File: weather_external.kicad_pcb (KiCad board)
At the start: 2 copper layers, 36 x 76 mm, 19 parts, among them J1 Conn_01x06_Male, J2 Conn_01x02_Male, J3 Conn_01x03_Male, J4 Conn_01x04_Male, Q1 IRF510PBF, SW1 SW_Push, U1 MCP1700-3302E_SOT23, U3 NE555DR

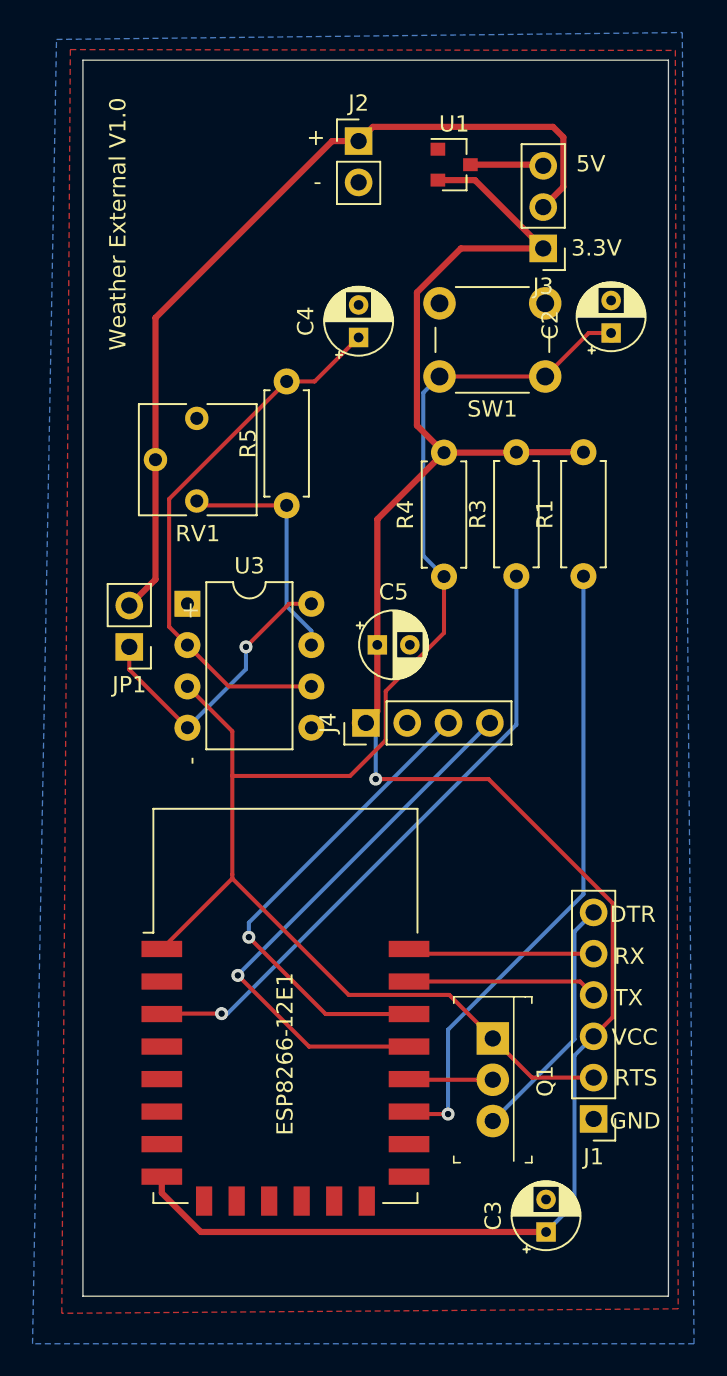
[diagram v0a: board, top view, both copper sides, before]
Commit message: Version 1.2. Small components
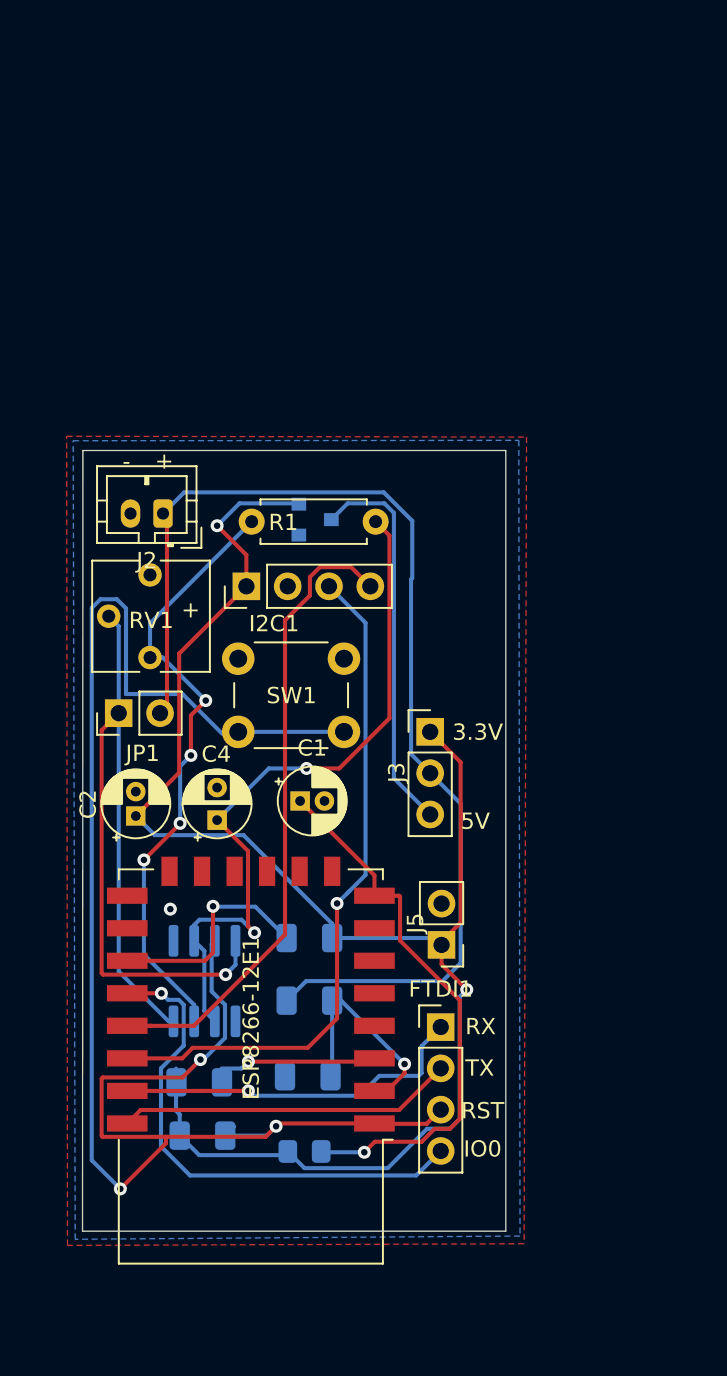
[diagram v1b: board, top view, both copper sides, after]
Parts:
- removed C3, C5: 0.1uF, Capacitor_THT:CP_Radial_D4.0mm_P2.00mm
- removed J1: Conn_01x06_Male, Connector_PinHeader_2.54mm:PinHeader_1x06_P2.54mm_Vertical
- removed Q1: IRF510PBF, digikey-footprints:TO-220-3
- removed the R1 at (29.8, 56.7)
- added C1: 0.1uf, Capacitor_THT:CP_Radial_D4.0mm_P1.50mm, F.Cu at (12.3, 70.5)
- added FTDI1: Conn_01x04_Male, Connector_PinHeader_2.54mm:PinHeader_1x04_P2.54mm_Vertical, F.Cu at (21.0, 84.5)
- added J5: Conn_01x02_Male, Connector_PinHeader_2.54mm:PinHeader_1x02_P2.54mm_Vertical, F.Cu at (21.1, 79.4)
- added L1: INDUCTOR, Inductor_SMD:L_0805_2012Metric_Pad1.15x1.40mm_HandSolder, B.Cu at (12.6, 92.1)
- added R2: 10k, Resistor_SMD:R_1206_3216Metric, B.Cu at (6.35, 91.1)
- added R5: 100k, Resistor_SMD:R_1206_3216Metric, B.Cu at (12.9, 82.8)
- added R6: 270k, Resistor_SMD:R_1206_3216Metric, B.Cu at (12.8, 87.5)
- C2: value 220uF -> 47uf; footprint Capacitor_THT:CP_Radial_D4.0mm_P2.00mm -> Capacitor_THT:CP_Radial_D4.0mm_P1.50mm
- J2: footprint Connector_PinHeader_2.54mm:PinHeader_1x02_P2.54mm_Vertical -> Connector_JST:JST_PH_B2B-PH-K_1x02_P2.00mm_Vertical
- R3, R4: footprint Resistor_THT:R_Axial_DIN0207_L6.3mm_D2.5mm_P7.62mm_Horizontal -> Resistor_SMD:R_1206_3216Metric; moved to B.Cu
- U1: moved to B.Cu
- U3: footprint Package_DIP:DIP-8_W7.62mm -> Package_SO:SOIC-8_3.9x4.9mm_P1.27mm; moved to B.Cu
- moved C2 41.7 mm to (2.25, 71.5)
- moved R3 36.7 mm to (6.15, 87.8), turned to 0 degrees
- moved C4 30.9 mm to (7.25, 71.7)
- moved J3 30.5 mm to (20.4, 66.3), turned to 0 degrees
- moved J2 25.9 mm to (3.92, 52.9), turned to 180 degrees
- moved SW1 25.1 mm to (15.1, 66.3)
- moved R4 23.7 mm to (12.9, 79.0), turned to 180 degrees
- moved U1 23.4 mm to (13.3, 53.2)
- moved U3 23.2 mm to (6.47, 81.6), turned to 270 degrees
- moved I2C1 11.2 mm to (9.05, 57.4)
- moved RV1 10.0 mm to (3.12, 56.6)
- moved ESP8266-12E1 4.29 mm to (9.32, 86.9), turned to 180 degrees
- moved JP1 4.13 mm to (1.20, 65.2), turned to 90 degrees
- moved R1 2.37 mm to (9.38, 53.4), turned to 0 degrees
- renumbered J4 to I2C1, R5 to R1
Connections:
- C2 pad 1: Net-(C2-Pad1) -> +3V3
- ESP8266-12E1 pad 1: Net-(C2-Pad1) -> Net-(ESP8266-12E1-Pad1)
- ESP8266-12E1 pad 2: (no net) -> Net-(ESP8266-12E1-Pad2)
- ESP8266-12E1 pad 8: Net-(C3-Pad1) -> Net-(C1-Pad1)
- I2C1 pad 1: Net-(C3-Pad1) -> +3V3
- J3 pad 1: Net-(C3-Pad1) -> +3V3
- R3 pad 1: Net-(ESP8266-12E1-Pad3) -> +3V3
- R3 pad 2: Net-(C3-Pad1) -> Net-(ESP8266-12E1-Pad3)
- R4 pad 1: Net-(C2-Pad1) -> +3V3
- R4 pad 2: Net-(C3-Pad1) -> Net-(ESP8266-12E1-Pad17)
- RV1 pad 2: VCC -> Net-(JP1-Pad1)
- SW1 pad 1: Net-(C2-Pad1) -> Net-(ESP8266-12E1-Pad1)
- U1 pad 2: Net-(C3-Pad1) -> +3V3
- U3 pad 3: Net-(C2-Pad1) -> Net-(ESP8266-12E1-Pad1)
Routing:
- net Net-(C3-Pad1): track 124.6 -> 0.00 mm, vias 1 -> 0
- net Net-(ESP8266-12E1-Pad1): track 0.00 -> 106.9 mm, vias 0 -> 3
- net +3V3: track 0.00 -> 99.2 mm, vias 0 -> 2
- net Net-(C2-Pad1): track 94.3 -> 0.00 mm
- net Net-(JP1-Pad1): track 18.1 -> 53.1 mm
- net Net-(C1-Pad1): track 0.00 -> 33.9 mm, vias 0 -> 1
- net Net-(ESP8266-12E1-Pad3): track 38.5 -> 9.66 mm
- net Net-(ESP8266-12E1-Pad18): track 5.17 -> 31.6 mm, vias 0 -> 1
- net Net-(ESP8266-12E1-Pad17): track 39.0 -> 13.7 mm
- net Net-(R1-Pad1): track 14.9 -> 38.0 mm, vias 0 -> 4
- net Net-(J3-Pad3): track 4.50 -> 24.0 mm
- net VCC: track 53.6 -> 69.6 mm
- net Net-(J1-Pad6): track 15.4 -> 0.00 mm
- net Net-(ESP8266-12E1-Pad2): track 0.00 -> 15.0 mm, vias 0 -> 1
- net Net-(ESP8266-12E1-Pad20): track 30.1 -> 42.4 mm
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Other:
- board size 36 x 76 mm -> 26 x 48 mm
- board text added: "IO0"
- board text added: "RST"
- board text added: "Weather External V1.2"
- board text removed: "555 on/off"
- board text removed: "DTR"
- board text removed: "FTDI"
- board text removed: "GND"
- board text removed: "RTS"
- board text removed: "VCC"
- board text removed: "Weather External V1.0"
